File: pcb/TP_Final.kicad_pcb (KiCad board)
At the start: 2 copper layers, 20 parts, among them J1 A, J2 B, Q1 DMN2058U, U1 MQ-137, U2 MCP3551, U3 TXB0106

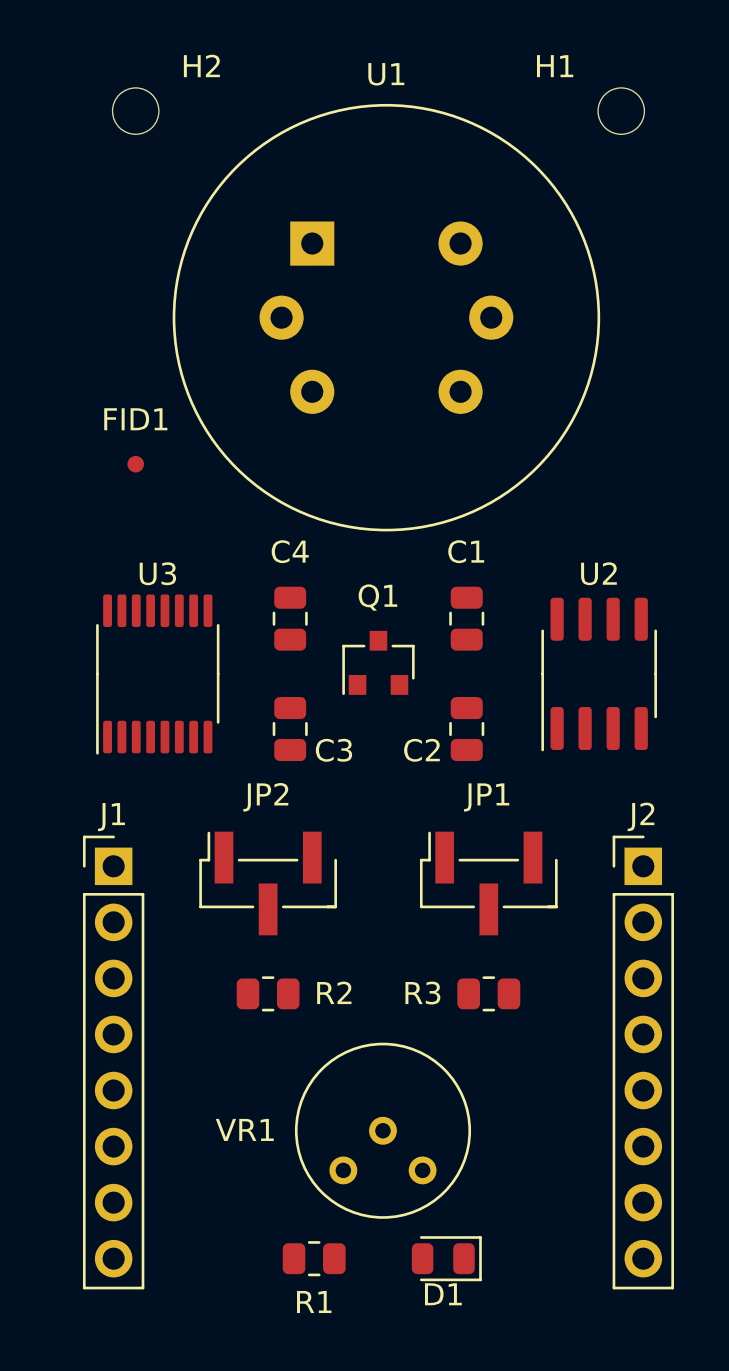
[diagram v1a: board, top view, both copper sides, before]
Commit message: Actualizo PCB
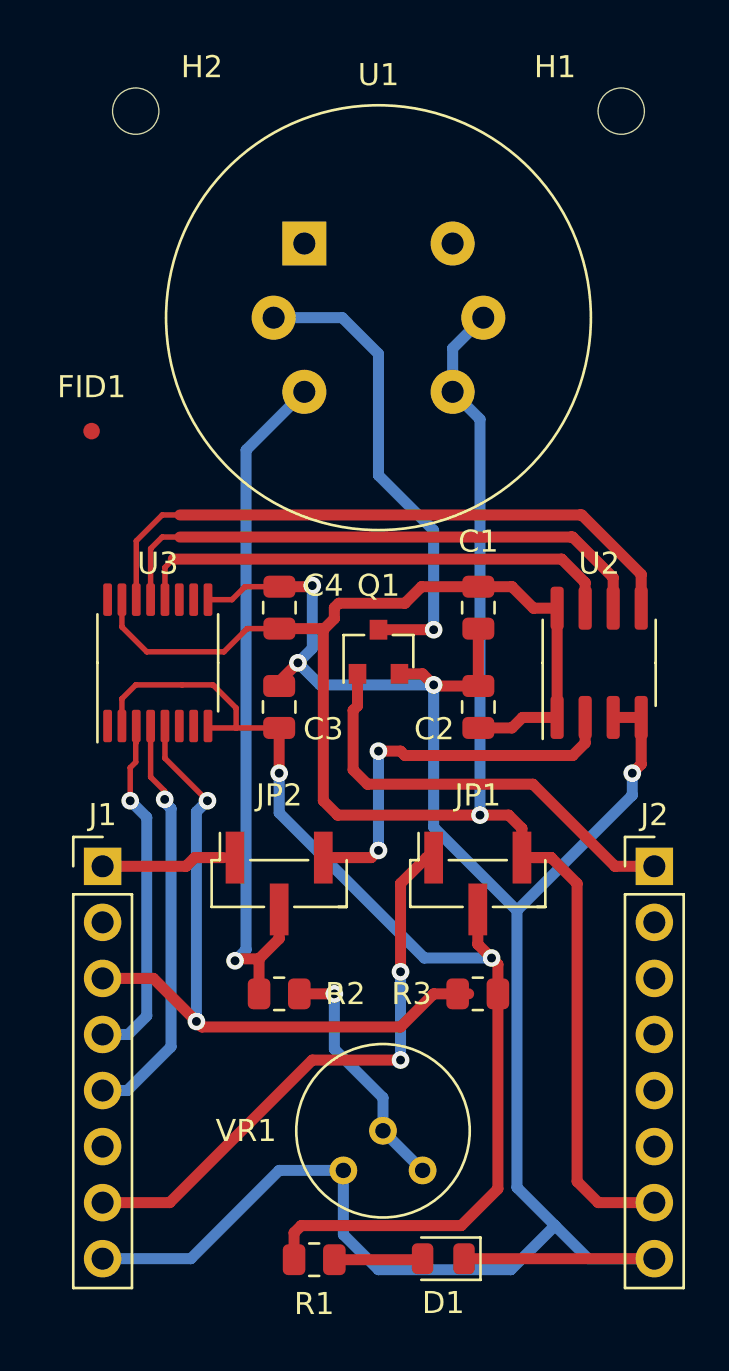
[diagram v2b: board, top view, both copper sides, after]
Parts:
- moved FID1 2.50 mm to (102.0, 88.5)
- moved C2 1.13 mm to (119.5, 101.0)
- moved C3 1.12 mm to (110.5, 101.0)
- moved C1 0.73 mm to (119.5, 96.5)
- moved C4 0.70 mm to (110.5, 96.5), turned to 90 degrees
- moved J1 0.50 mm to (102.5, 108.2)
- moved J2 0.50 mm to (127.5, 108.2)
- moved JP1 0.50 mm to (119.5, 109.0)
- moved JP2 0.50 mm to (110.5, 109.0)
- moved Q1 0.50 mm to (115.0, 98.5)
- moved R2 0.50 mm to (110.5, 114.0)
- moved R3 0.50 mm to (119.5, 114.0)
- moved U2 0.50 mm to (125.0, 99.0)
- moved U3 0.50 mm to (105.0, 99.0)
- moved U1 0.36 mm to (111.6, 80.0)
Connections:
- J1 pad 2: /NC -> Net-(J1-Pad2)
- J1 pad 6: /NC -> Net-(J1-Pad6)
- J2 pad 2: /NC -> Net-(J2-Pad2)
- J2 pad 3: /NC -> Net-(J2-Pad3)
- J2 pad 4: /NC -> Net-(J2-Pad4)
- J2 pad 5: /NC -> Net-(J2-Pad5)
- J2 pad 6: /NC -> Net-(J2-Pad6)
- U1 pad 1: Net-(JP2-Pad2) -> Net-(U1-Pad1)
- U1 pad 2: +5V -> Net-(Q1-Pad3)
- U1 pad 3: Net-(U1-Pad3) -> Net-(JP2-Pad2)
- U1 pad 4: Net-(U1-Pad4) -> +5V
- U1 pad 5: Net-(Q1-Pad3) -> +5V
- U1 pad 6: +5V -> Net-(U1-Pad6)
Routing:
- net GND: track 0.00 -> 102.6 mm, vias 0 -> 4
- net +5V: track 0.00 -> 96.1 mm, vias 0 -> 1
- net VCC: track 0.00 -> 51.8 mm, vias 0 -> 2
- net Net-(JP2-Pad2): track 0.00 -> 32.4 mm, vias 0 -> 1
- net /CS: track 0.00 -> 32.0 mm, vias 0 -> 2
- net /!SCK: track 0.00 -> 28.7 mm
- net +3V3: track 0.00 -> 25.7 mm, vias 0 -> 2
- net /!MISO: track 0.00 -> 25.6 mm
- net /!CS: track 0.00 -> 22.3 mm
- net Net-(Q1-Pad3): track 0.00 -> 21.5 mm, vias 0 -> 1
- net /PWM: track 0.00 -> 19.9 mm
- net /MISO: track 0.00 -> 18.8 mm, vias 0 -> 1
- net /ADC: track 0.00 -> 18.0 mm, vias 0 -> 2
- net /SCK: track 0.00 -> 15.9 mm, vias 0 -> 1
- net Net-(R2-Pad2): track 0.00 -> 11.2 mm, vias 0 -> 1
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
